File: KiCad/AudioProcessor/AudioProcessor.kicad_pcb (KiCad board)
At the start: 2 copper layers, 56 x 43 mm, 49 parts, among them J1 IN4, J2 IN3, J3 IN2, J4 IN1, J5 AUX, J6 I2C, J7 LOUT, J8 ROUT, J9 POWER, U1 TDA7440

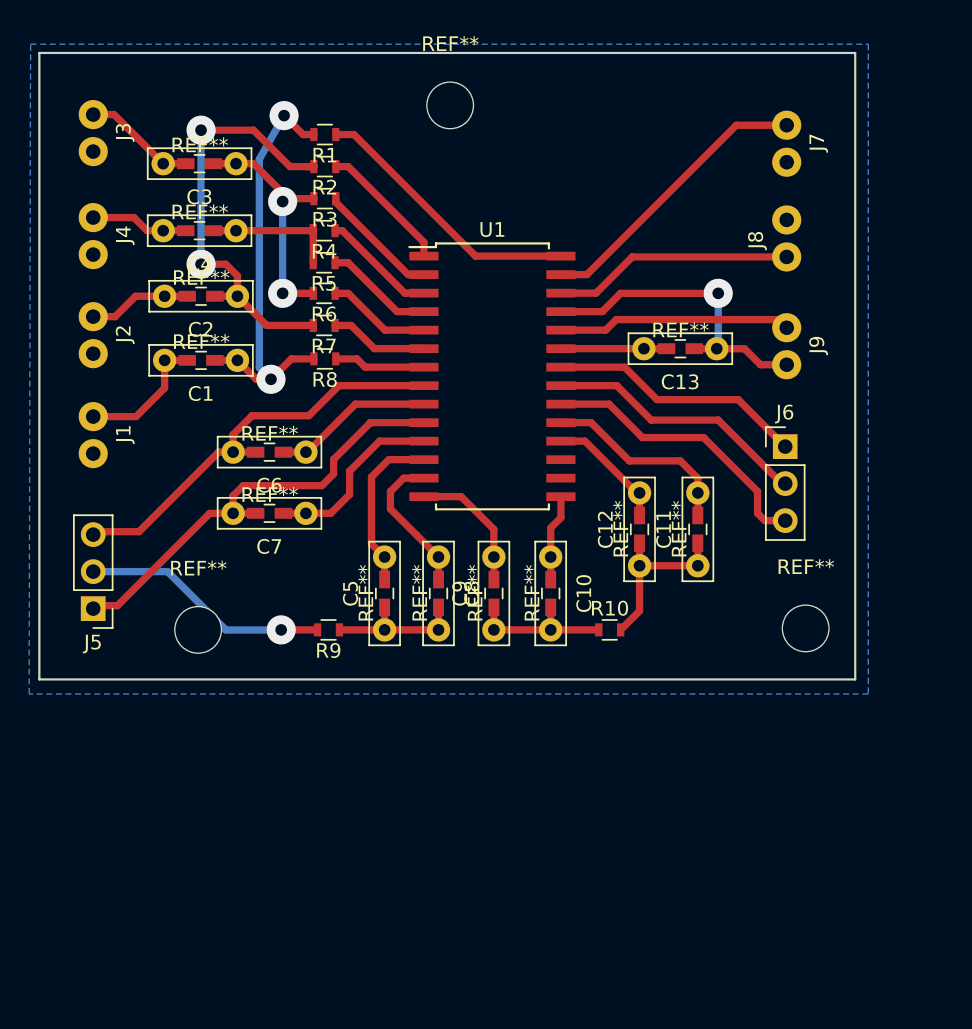
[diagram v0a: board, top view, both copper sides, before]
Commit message: Audio processor PCB is ready
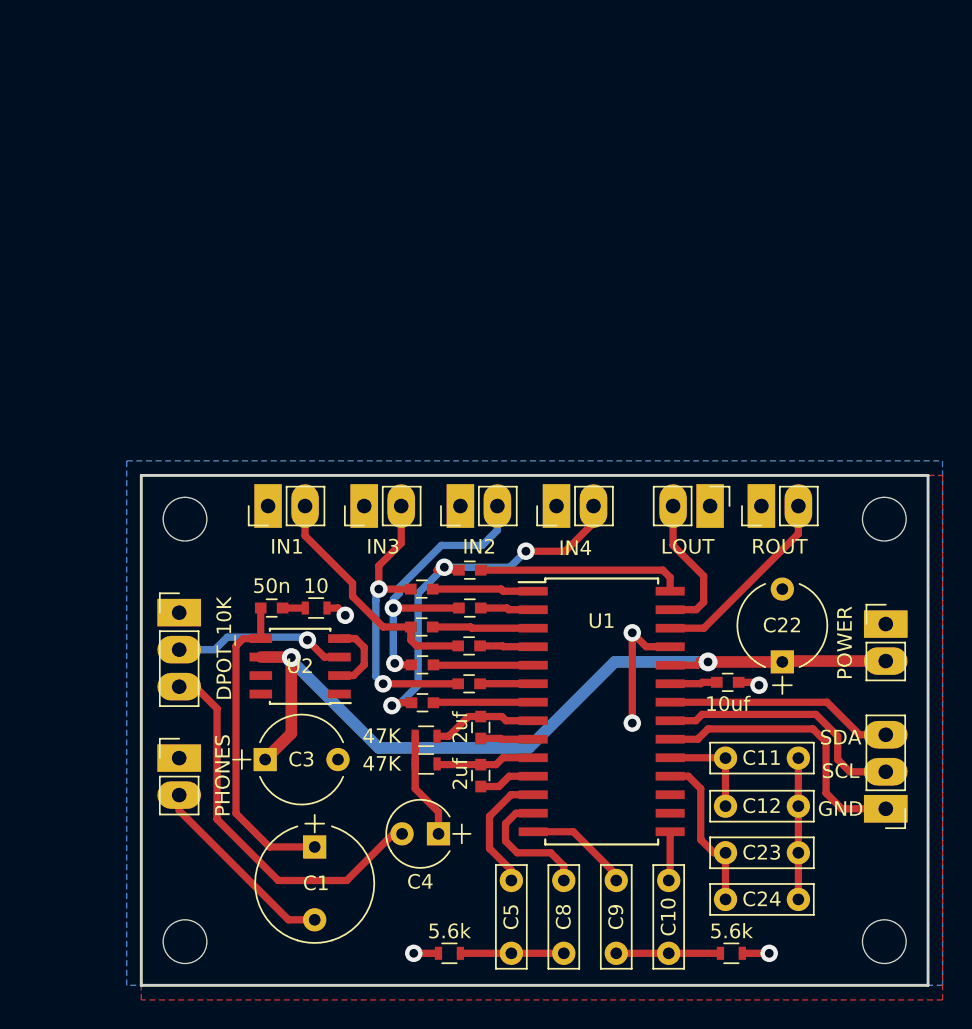
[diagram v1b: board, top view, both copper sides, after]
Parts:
- removed R4, R5, R6, R7, R8: 600, Resistors_SMD:R_0603
- removed the REF** at (134.0, 71.3)
- removed the REF** at (101.1, 72.1)
- removed the REF** at (101.1, 67.7)
- removed the REF** at (101.0, 63.2)
- removed the REF** at (101.0, 58.6)
- removed the REF** at (118.2, 54.6)
- removed the REF** at (142.6, 90.5)
- removed the REF** at (100.9, 90.6)
- removed the REF** at (135.2, 83.7)
- removed the REF** at (131.2, 83.7)
- removed the REF** at (125.1, 88.1)
- removed the REF** at (121.2, 88.1)
- removed the REF** at (117.4, 88.1)
- removed the REF** at (113.7, 88.1)
- removed the REF** at (105.8, 82.6)
- removed the REF** at (105.8, 78.4)
- added C14: 2uf, Capacitors_SMD:C_0603, F.Cu at (119.5, 86.5)
- added C15: 2uf, Capacitors_SMD:C_0603, F.Cu at (119.5, 89.1)
- added C16: 2uf, Capacitors_SMD:C_0603, F.Cu at (119.5, 91.7)
- added C17: 2uf, Capacitors_SMD:C_0603, F.Cu at (119.5, 94.3)
- added C18: 2uf, Capacitors_SMD:C_0603, F.Cu at (116.2, 87.8)
- added C19: 2uf, Capacitors_SMD:C_0603, F.Cu at (116.2, 90.4)
- added C20: 2uf, Capacitors_SMD:C_0603, F.Cu at (116.3, 93.0)
- added C21: 2uf, Capacitors_SMD:C_0603, F.Cu at (116.3, 95.6)
- added C22: 100uf, Capacitors_THT:CP_Radial_Tantal_D6.0mm_P5.00mm, F.Cu at (141.0, 92.8)
- added C23: 4.7n, Capacitors_THT:C_Rect_L7.0mm_W2.0mm_P5.00mm, F.Cu at (142.1, 105.9)
- added C24: 1n, Capacitors_THT:C_Rect_L7.0mm_W2.0mm_P5.00mm, F.Cu at (142.1, 109.1)
- added J10: DPOT_10K, KiCadCustomLibs:Conn_1x03_2.54mm, F.Cu at (99.6, 89.4)
- added REF**: MountingHole_3mm, Mounting_Holes:MountingHole_3mm, F.Cu at (148.0, 112.0)
- added REF**: MountingHole_3mm, Mounting_Holes:MountingHole_3mm, F.Cu at (100.0, 112.0)
- added REF**: MountingHole_3mm, Mounting_Holes:MountingHole_3mm, F.Cu at (100.0, 83.0)
- added REF**: MountingHole_3mm, Mounting_Holes:MountingHole_3mm, F.Cu at (148.0, 83.0)
- added U2: LM386M, Housings_SOIC:SOIC-8_3.9x4.9mm_Pitch1.27mm, F.Cu at (107.9, 93.1)
- C1: value 2.2uf -> 220uf; footprint Capacitors_THT:C_Rect_L7.0mm_W2.0mm_P5.00mm -> Capacitors_THT:CP_Radial_Tantal_D8.0mm_P5.00mm
- C11: value 5.6n -> 4.7n
- C12: value 5.6n -> 1n
- C13: value 2.2uf -> 10uf; footprint Capacitors_THT:C_Rect_L7.0mm_W2.0mm_P5.00mm -> Capacitors_SMD:C_0603
- C2: value 2.2uf -> 50n; footprint Capacitors_THT:C_Rect_L7.0mm_W2.0mm_P5.00mm -> Capacitors_SMD:C_0603
- C3: value 2.2uf -> 100uf; footprint Capacitors_THT:C_Rect_L7.0mm_W2.0mm_P5.00mm -> Capacitors_THT:CP_Radial_Tantal_D6.0mm_P5.00mm
- C4: value 2.2uf -> 10uf; footprint Capacitors_THT:C_Rect_L7.0mm_W2.0mm_P5.00mm -> Capacitors_THT:CP_Radial_Tantal_D4.5mm_P2.50mm
- C6, C7: value 2.2uf -> 2uf; footprint Capacitors_THT:C_Rect_L7.0mm_W2.0mm_P5.00mm -> Capacitors_SMD:C_0603
- J1, J2, J3, J4, J7, J8, J9: footprint KiCadCustomLibs:Conn2pin_2.54mm -> KiCadCustomLibs:Conn_1x02_2.54mm
- J5: value AUX -> PHONES; footprint Pin_Headers:Pin_Header_Straight_1x03_Pitch2.54mm -> KiCadCustomLibs:Conn_1x02_2.54mm
- J6: footprint Pin_Headers:Pin_Header_Straight_1x03_Pitch2.54mm -> KiCadCustomLibs:Conn_1x03_2.54mm
- R1: value 600 -> 10
- R2, R3: value 600 -> 47K
- moved C4 43.7 mm to (117.4, 104.6)
- moved C3 40.9 mm to (105.5, 99.5), turned to 0 degrees
- moved R2 39.7 mm to (116.5, 97.9)
- moved R3 39.4 mm to (116.5, 99.8)
- moved J3 35.9 mm to (118.9, 82.1), turned to 90 degrees
- moved C1 33.8 mm to (108.9, 105.5), turned to 270 degrees
- moved R1 32.5 mm to (109.0, 89.1), turned to 0 degrees
- moved J1 32.2 mm to (125.5, 82.1), turned to 90 degrees
- moved J6 25.8 mm to (148.1, 102.9), turned to 180 degrees
- moved J7 25.4 mm to (136.0, 82.1)
- moved U1 24.2 mm to (128.6, 96.2)
- moved C5 23.8 mm to (122.4, 112.8)
- moved C8 23.8 mm to (126.0, 107.8)
- moved C9 23.7 mm to (129.6, 112.8)
- moved R10 23.7 mm to (137.5, 112.8)
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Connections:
- C1 pad 2: /IN4 -> Net-(C1-Pad2)
- C12 pad 2: Net-(C12-Pad2) -> Net-(C11-Pad2)
- C2 pad 2: /IN3 -> Net-(C1-Pad1)
- C3 pad 1: Net-(C3-Pad1) -> +9V
- C3 pad 2: /IN2 -> GNDA
- C4 pad 2: /IN1 -> /AUX
- J1 pad 1: /IN4 -> GNDA
- J1 pad 2: GNDA -> /IN4
- J2 pad 1: /IN3 -> GNDA
- J2 pad 2: GNDA -> /IN3
- J3 pad 1: /IN2 -> GNDA
- J3 pad 2: GNDA -> /IN2
- J4 pad 1: /IN1 -> GNDA
- J4 pad 2: GNDA -> /IN1
- J5 pad 1: Net-(C7-Pad2) -> GNDA
- J5 pad 2: GNDA -> Net-(C1-Pad2)
- J6 pad 1: /SDA -> /GND
- J6 pad 3: GND -> /SDA
- J7 pad 1: /LOUT -> GNDA
- J7 pad 2: GNDA -> /LOUT
- J8 pad 1: /ROUT -> GNDA
- J8 pad 2: GNDA -> /ROUT
- J9 pad 1: +9V -> GNDA
- J9 pad 2: GNDA -> +9V
- R1 pad 1: Net-(R1-Pad1) -> Net-(C2-Pad1)
- R1 pad 2: Net-(C1-Pad1) -> GNDA
- R2 pad 1: Net-(R2-Pad1) -> Net-(C6-Pad2)
- R2 pad 2: Net-(C2-Pad1) -> Net-(C4-Pad1)
- R3 pad 1: Net-(R3-Pad1) -> Net-(C7-Pad2)
- R3 pad 2: Net-(C3-Pad1) -> Net-(C4-Pad1)
- U1 pad 1: Net-(R2-Pad1) -> Net-(C18-Pad1)
- U1 pad 18: Net-(C12-Pad2) -> Net-(C23-Pad2)
- U1 pad 2: Net-(R3-Pad1) -> Net-(C15-Pad1)
- U1 pad 20: GND -> /GND
- U1 pad 28: Net-(R1-Pad1) -> Net-(C14-Pad1)
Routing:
- net +9V: track 16.0 -> 58.5 mm, vias 0 -> 2
- net Net-(C2-Pad1): track 30.5 -> 1.55 mm, vias 2 -> 0
- net /AUX: track 0.00 -> 26.6 mm
- net Net-(C7-Pad2): track 30.8 -> 6.82 mm
- net Net-(C6-Pad2): track 29.2 -> 7.28 mm
- net GNDA: track 51.1 -> 30.5 mm, vias 2 -> 6
- net GND: track 19.6 -> 0.00 mm
- net /GND: track 0.00 -> 19.4 mm
- net Net-(R1-Pad1): track 18.9 -> 0.00 mm
- net /IN4: track 9.16 -> 27.4 mm, vias 0 -> 3
- net Net-(C3-Pad1): track 16.8 -> 0.00 mm, vias 2 -> 0
- net Net-(C14-Pad1): track 0.00 -> 14.2 mm
- net Net-(C1-Pad2): track 0.00 -> 13.5 mm
- net /IN3: track 7.03 -> 20.5 mm, vias 0 -> 2
- net /IN2: track 7.75 -> 21.1 mm, vias 0 -> 2
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- added copper zone on F.Cu, net GNDA
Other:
- board size 56 x 43 mm -> 54 x 35 mm
- net class Default: via_dia 2 -> 1.2; via_drill 0.8 -> 0.6
- net class PWR added: clearance 0.3, trace_width 0.8, via_dia 1.3, via_drill 0.6
- board text added: "+"
- board text added: "-"
- board text added: "9V"
- board text added: "GND"
- board text added: "NPPC 2019"
- board text added: "SCL"
- board text added: "SDA"
- board text added: "TDA7440 Audio Processor"
